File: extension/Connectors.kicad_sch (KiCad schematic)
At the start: 2 parts, among them X701 MB2, X702 MB1

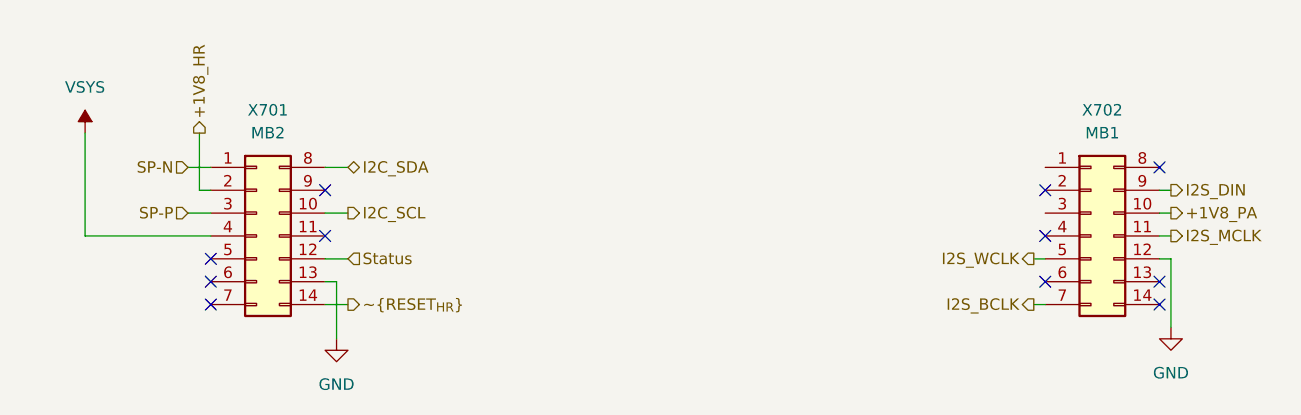
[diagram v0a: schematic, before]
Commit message: Prepare release 1.0.0
Signed-off-by: Daniel Kampert <danielkampert@kampis-elektroecke.de>
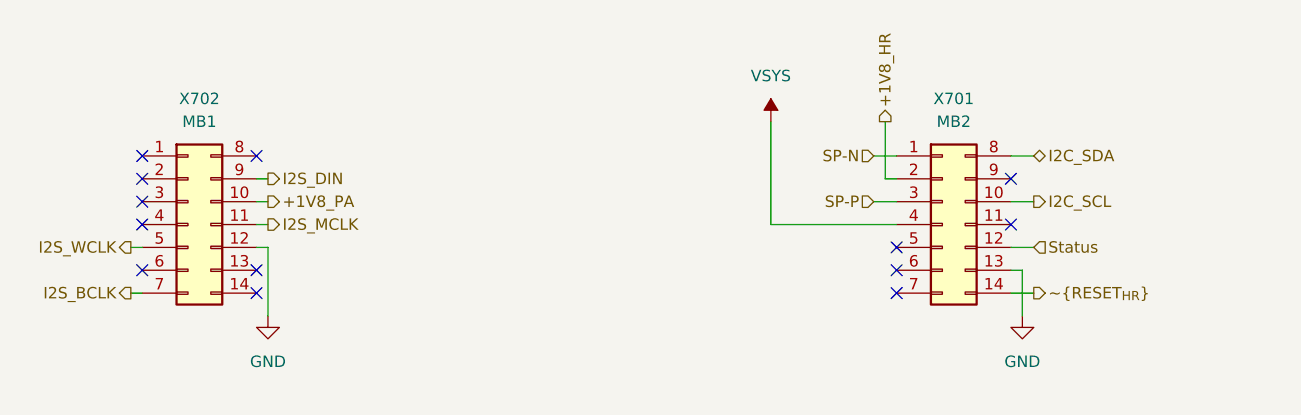
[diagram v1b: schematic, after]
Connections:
- no-connect marks 11 -> 13
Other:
- title: Connectors -> (none)
- moved on the sheet: X701, X702
